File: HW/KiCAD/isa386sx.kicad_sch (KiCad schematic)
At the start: 174 parts, among them CON1 CF-CARD-cfcard, J10 PC104_16, J11 PC104, J12 USB_B, J13 POWER 5V2A, J14 COM1, J15 COM2, J16 ESP, J17 Mini-DIN-6, J18 Mini-DIN-6, J9 Conn_01x04, Q1 BC817, Q2 BC856, Q3 BC856, SW1 Jumper / Pin header 1x2 Pitch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, SW2 SW_Push, SW3 SW_DIP_x01, U10 74HCT32PW, U11 MSM5118160F-JS, U12 74HCT138PW, U13 ST16C554D, U14 74HCT138PW, U15 GD75232PW, U16 GD75232PW, U17 MAX809LEUR, U18 CH340G, U19 LMR62014, U20 ESP-12F, U21 IP4220CZ6, U22 IP4220CZ6, U23 1117-3.3, U24 ICL7660A, U25 39SF040, U26 TXS0104PW, U6 MSM5118160F-JS, U7 M6117D, U8 MSM5118160F-JS, U9 MSM5118160F-JS, X1 14.318 MHz, X2 80 MHz, X3 1.8432 Mhz, Y3 32768 Hz, Y4 12 MHz

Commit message: some edit
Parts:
- BT1: footprint my:CR2032V -> Battery:BatteryHolder_MYOUNG_BS-07-A1BJ001_CR2032
- C102, C103, C98: footprint Capacitor_Tantalum_SMD:CP_EIA-3528-21_Kemet-B_Pad1.50x2.35mm_HandSolder -> Capacitor_Tantalum_SMD:CP_EIA-3528-21_Kemet-B_HandSolder
- C75: footprint Capacitor_Tantalum_SMD:CP_EIA-7343-31_Kemet-D_Pad2.25x2.55mm_HandSolder -> Capacitor_Tantalum_SMD:CP_EIA-7343-31_Kemet-D_HandSolder
- CON1: footprint my:TE_1734451-1-LONG -> Library:TE_1734451-1
- H1, H2, H3, H4: footprint my:MountingHole_3.2mm_M3_dk5.2mm_Mask -> Library_user:MountingHole_3.2mm_M3_dk5.2mm_Mask
- J17, J18: footprint my:minidin-6 -> Library_user:minidin-6
- LOGO1: footprint mygraphic:black-mage-12.5x8.6 -> Library_user:black-mage-12.5x8.6
- U11, U6, U8, U9: footprint my:SOJ-42 -> Library_user:SOJ-42
- U25: footprint my:PLCC-32_11.4x14.0mm_P1.27mm-longpads -> Library_user:PLCC-32_11.4x14.0mm_P1.27mm-longpads
- X1, X2: footprint my:Oscillator_SMD_7050_7.0x5.0mm -> Oscillator:Oscillator_SMD_Abracon_ASE-4Pin_3.2x2.5mm_HandSoldering
- X3: footprint my:Oscillator_SMD_7050_7.0x5.0mm -> Oscillator:Oscillator_SMD_Abracon_ASV-4Pin_7.0x5.1mm_HandSoldering
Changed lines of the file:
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@@
 			)
 		)
-		(property "Footprint" "my:TE_1734451-1-LONG"
+		(property "Footprint" "Library:TE_1734451-1"
 			(at 233.172 69.85 0)
 			(effects
@@
 			)
 		)
-		(property "Footprint" "my:PLCC-32_11.4x14.0mm_P1.27mm-longpads"
+		(property "Footprint" "Library_user:PLCC-32_11.4x14.0mm_P1.27mm-longpads"
 			(at 542.29 236.22 0)
 			(effects
@@
 			)
 		)
-		(property "Footprint" "Capacitor_Tantalum_SMD:CP_EIA-7343-31_Kemet-D_Pad2.25x2.55mm_HandSolder"
+		(property "Footprint" "Capacitor_Tantalum_SMD:CP_EIA-7343-31_Kemet-D_HandSolder"
 			(at 411.1752 -17.78 0)
 			(effects
@@
 			)
 		)
-		(property "Footprint" "my:CR2032V"
+		(property "Footprint" "Battery:BatteryHolder_MYOUNG_BS-07-A1BJ001_CR2032"
 			(at 566.42 40.386 90)
 			(effects
@@
 			)
 		)
-		(property "Footprint" "my:SOJ-42"
+		(property "Footprint" "Library_user:SOJ-42"
 			(at 137.16 358.14 0)
 			(effects
@@
 			)
 		)
-		(property "Footprint" "my:MountingHole_3.2mm_M3_dk5.2mm_Mask"
+		(property "Footprint" "Library_user:MountingHole_3.2mm_M3_dk5.2mm_Mask"
 			(at 552.45 293.37 0)
 			(effects
@@
 			)
 		)
-		(property "Footprint" "my:MountingHole_3.2mm_M3_dk5.2mm_Mask"
+		(property "Footprint" "Library_user:MountingHole_3.2mm_M3_dk5.2mm_Mask"
 			(at 552.45 298.45 0)
 			(effects
@@
 			)
 		)
-		(property "Footprint" "my:MountingHole_3.2mm_M3_dk5.2mm_Mask"
+		(property "Footprint" "Library_user:MountingHole_3.2mm_M3_dk5.2mm_Mask"
 			(at 552.45 303.53 0)
 			(effects
@@
 			)
 		)
-		(property "Footprint" "my:Oscillator_SMD_7050_7.0x5.0mm"
+		(property "Footprint" "Oscillator:Oscillator_SMD_Abracon_ASE-4Pin_3.2x2.5mm_HandSoldering"
 			(at 233.68 223.52 0)
 			(effects
@@
 			)
 		)
-		(property "Footprint" "Capacitor_Tantalum_SMD:CP_EIA-3528-21_Kemet-B_Pad1.50x2.35mm_HandSolder"
+		(property "Footprint" "Capacitor_Tantalum_SMD:CP_EIA-3528-21_Kemet-B_HandSolder"
 			(at 563.5752 90.17 0)
 			(effects
@@
 			)
 		)
-		(property "Footprint" "my:minidin-6"
+		(property "Footprint" "Library_user:minidin-6"
 			(at 560.07 171.45 0)
 			(effects
@@
 			)
 		)
-		(property "Footprint" "my:minidin-6"
+		(property "Footprint" "Library_user:minidin-6"
 			(at 560.07 133.35 0)
 			(effects
@@
 			)
 		)
-		(property "Footprint" "Capacitor_Tantalum_SMD:CP_EIA-3528-21_Kemet-B_Pad1.50x2.35mm_HandSolder"
+		(property "Footprint" "Capacitor_Tantalum_SMD:CP_EIA-3528-21_Kemet-B_HandSolder"
 			(at 540.7152 39.37 0)
 			(effects
@@
 			)
 		)
-		(property "Footprint" "my:MountingHole_3.2mm_M3_dk5.2mm_Mask"
+		(property "Footprint" "Library_user:MountingHole_3.2mm_M3_dk5.2mm_Mask"
 			(at 552.45 288.29 0)
 			(effects
@@
 			)
 		)
-		(property "Footprint" "my:Oscillator_SMD_7050_7.0x5.0mm"
+		(property "Footprint" "Oscillator:Oscillator_SMD_Abracon_ASE-4Pin_3.2x2.5mm_HandSoldering"
 			(at 233.68 199.39 0)
 			(effects
@@
 			)
 		)
-		(property "Footprint" "my:SOJ-42"
+		(property "Footprint" "Library_user:SOJ-42"
 			(at 260.35 358.14 0)
 			(effects
@@
 			)
 		)
-		(property "Footprint" "my:SOJ-42"
+		(property "Footprint" "Library_user:SOJ-42"
 			(at 73.66 358.14 0)
 			(effects
@@
 			)
 		)
-		(property "Footprint" "Capacitor_Tantalum_SMD:CP_EIA-3528-21_Kemet-B_Pad1.50x2.35mm_HandSolder"
+		(property "Footprint" "Capacitor_Tantalum_SMD:CP_EIA-3528-21_Kemet-B_HandSolder"
 			(at 555.9552 97.79 0)
 			(effects
@@
 			)
 		)
-		(property "Footprint" "my:Oscillator_SMD_7050_7.0x5.0mm"
+		(property "Footprint" "Oscillator:Oscillator_SMD_Abracon_ASV-4Pin_7.0x5.1mm_HandSoldering"
 			(at 309.88 276.86 0)
 			(effects
@@
 			)
 		)
-		(property "Footprint" "my:SOJ-42"
+		(property "Footprint" "Library_user:SOJ-42"
 			(at 196.85 358.14 0)
 			(effects
@@
 			)
 		)
-		(property "Footprint" "mygraphic:black-mage-12.5x8.6"
+		(property "Footprint" "Library_user:black-mage-12.5x8.6"
 			(at 523.24 301.625 0)
 			(effects

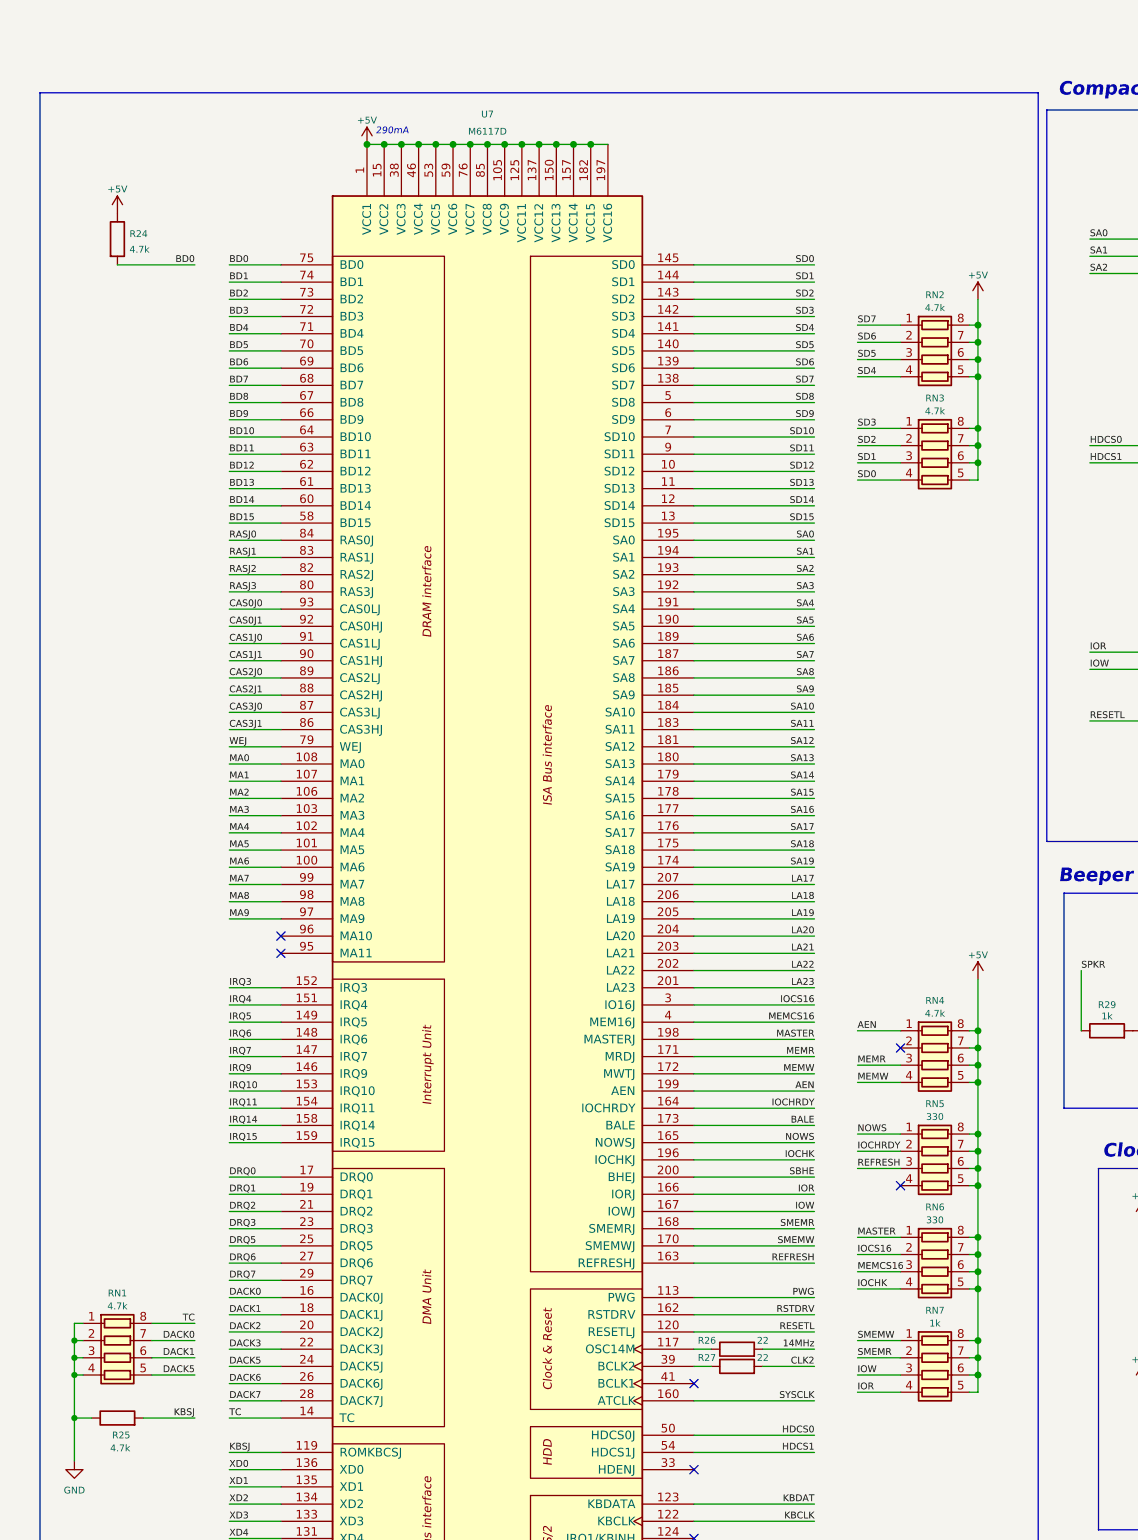
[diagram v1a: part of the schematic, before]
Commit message: pcb edit
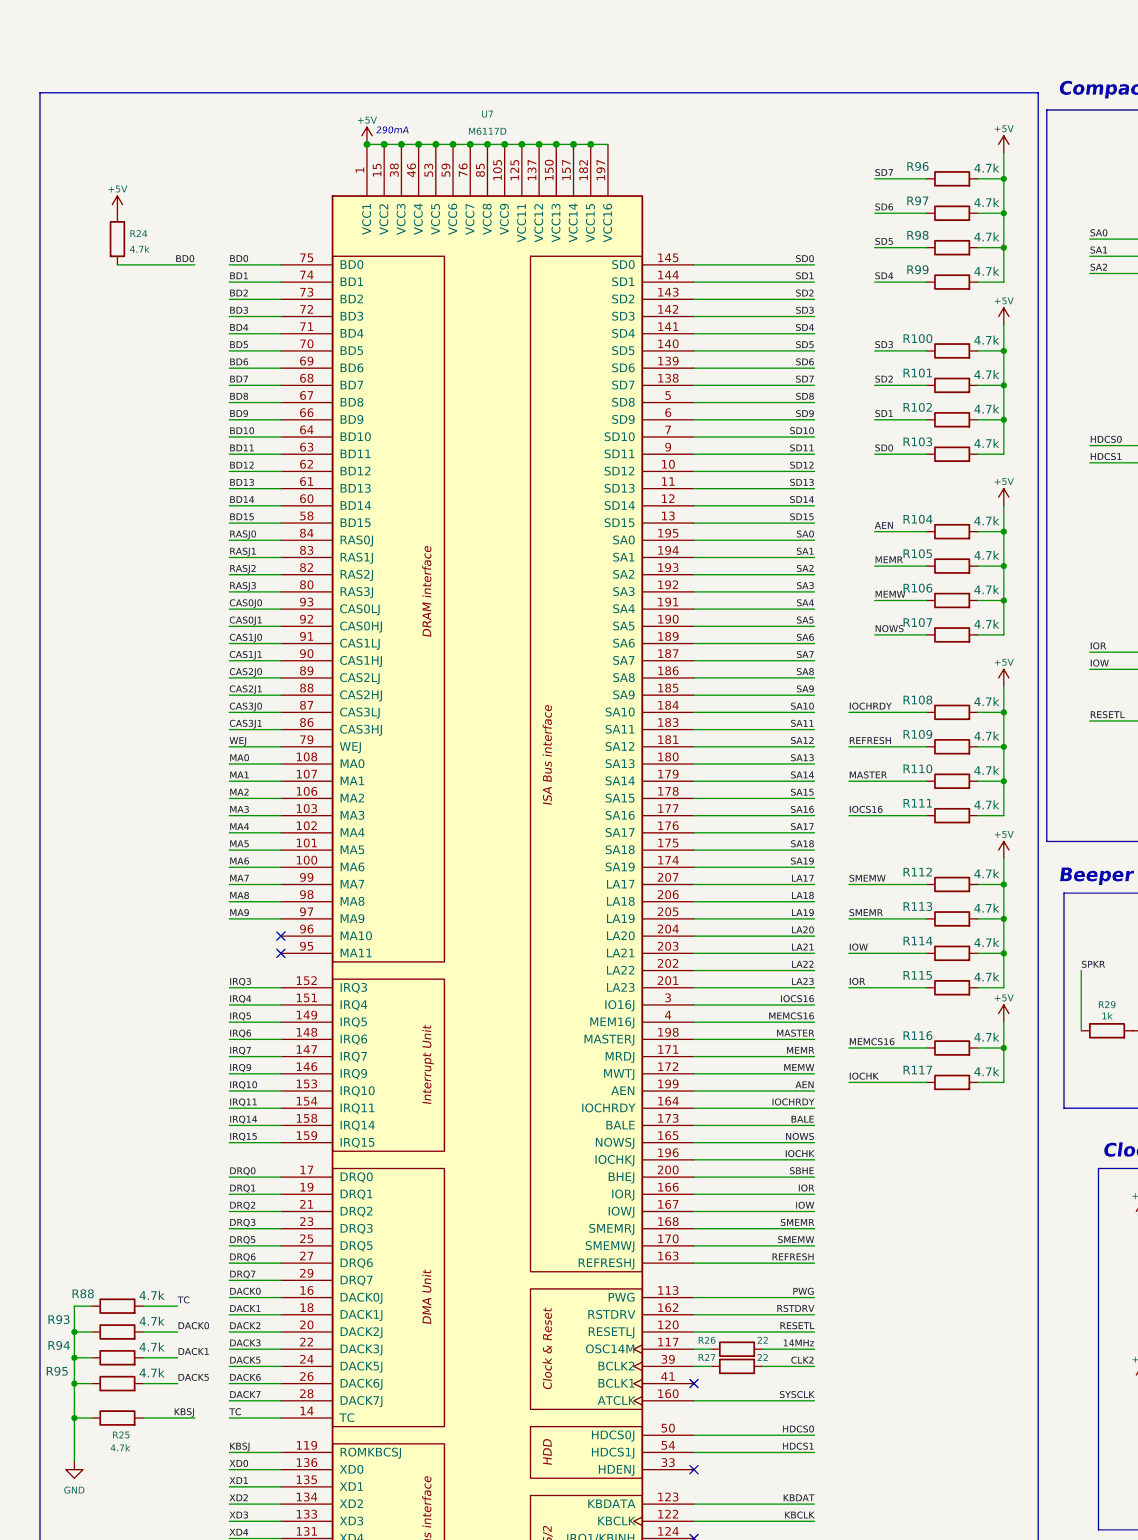
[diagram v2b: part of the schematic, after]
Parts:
- removed RN1, RN2, RN3, RN4: 4.7k, Resistor_SMD:R_Array_Convex_4x0603, symbol Device:R_Pack04
- removed RN5, RN6: 330, Resistor_SMD:R_Array_Convex_4x0603, symbol Device:R_Pack04
- removed RN7: 1k, Resistor_SMD:R_Array_Convex_4x0603, symbol Device:R_Pack04
- added R100, R101, R102, R103, R104, R105, R106, R107, R108, R109, R110, R111, R112, R113, R114, R115, R116, R117, R88, R93, R94, R95, R96, R97, R98, R99: 4.7k, Resistor_SMD:R_0805_2012Metric_Pad1.20x1.40mm_HandSolder, symbol Device:R
- C100, C101, C29, C30, C31, C33, C34, C35, C36, C37, C38, C39, C40, C41, C42, C43, C44, C45, C46, C47, C48, C49, C50, C51, C52, C53, C54, C55, C56, C57, C58, C59, C60, C61, C62, C63, C64, C65, C66, C67, C68, C69, C71, C73, C76, C77, C79, C80, C81, C82, C83, C85, C86, C87, C88, C90, C91, C92, C96, C97, C99: footprint Capacitor_SMD:C_0603_1608Metric_Pad1.08x0.95mm_HandSolder -> Capacitor_SMD:C_0805_2012Metric_Pad1.18x1.45mm_HandSolder
- L4: footprint Inductor_SMD:L_Taiyo-Yuden_NR-60xx_HandSoldering -> Inductor_SMD:L_Panasonic_PCC-M0850M
- R24, R25, R26, R27, R28, R29, R31, R32, R33, R34, R35, R36, R37, R38, R39, R40, R43, R44, R45, R46, R47, R48, R49, R50, R51, R52: footprint Resistor_SMD:R_0603_1608Metric_Pad0.98x0.95mm_HandSolder -> Resistor_SMD:R_0805_2012Metric_Pad1.20x1.40mm_HandSolder
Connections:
- net +5V: now also R100.2, R101.2, R102.2, R103.2, R104.2, R105.2, R106.2, R107.2, R108.2, R109.2, R110.2, R111.2, R112.2, R113.2, R114.2, R115.2, R116.2, R117.2, R96.2, R97.2, R98.2, R99.2
- net GND: now also R88.1, R93.1, R94.1, R95.1
- net IOCS16: now also R111.1
- net ISA_AEN: now also R104.1
- net ISA_DACK0: now also R93.2
- net ISA_DACK1: now also R94.2
- net ISA_DACK5: now also R95.2
- net ISA_IOCHK: now also R117.1
- net ISA_IOR: now also R115.1
- net ISA_IORDY: now also R108.1
- net ISA_IOW: now also R114.1
- net ISA_MASTER: now also R110.1
- net ISA_MEMCS16: now also R116.1
- net ISA_MEMR: now also R105.1
- net ISA_MEMW: now also R106.1
- net ISA_NOWS: now also R107.1
- net ISA_REFRESH: now also R109.1
- net ISA_SD0: now also R103.1
- net ISA_SD1: now also R102.1
- net ISA_SD2: now also R101.1
- net ISA_SD3: now also R100.1
- net ISA_SD4: now also R99.1
- net ISA_SD5: now also R98.1
- net ISA_SD6: now also R97.1
- net ISA_SD7: now also R96.1
- net ISA_SMEMR: now also R113.1
- net ISA_SMEMW: now also R112.1
- net ISA_TC: now also R88.2
- no-connect marks 80 -> 78
